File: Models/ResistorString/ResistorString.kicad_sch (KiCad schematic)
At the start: 3 parts

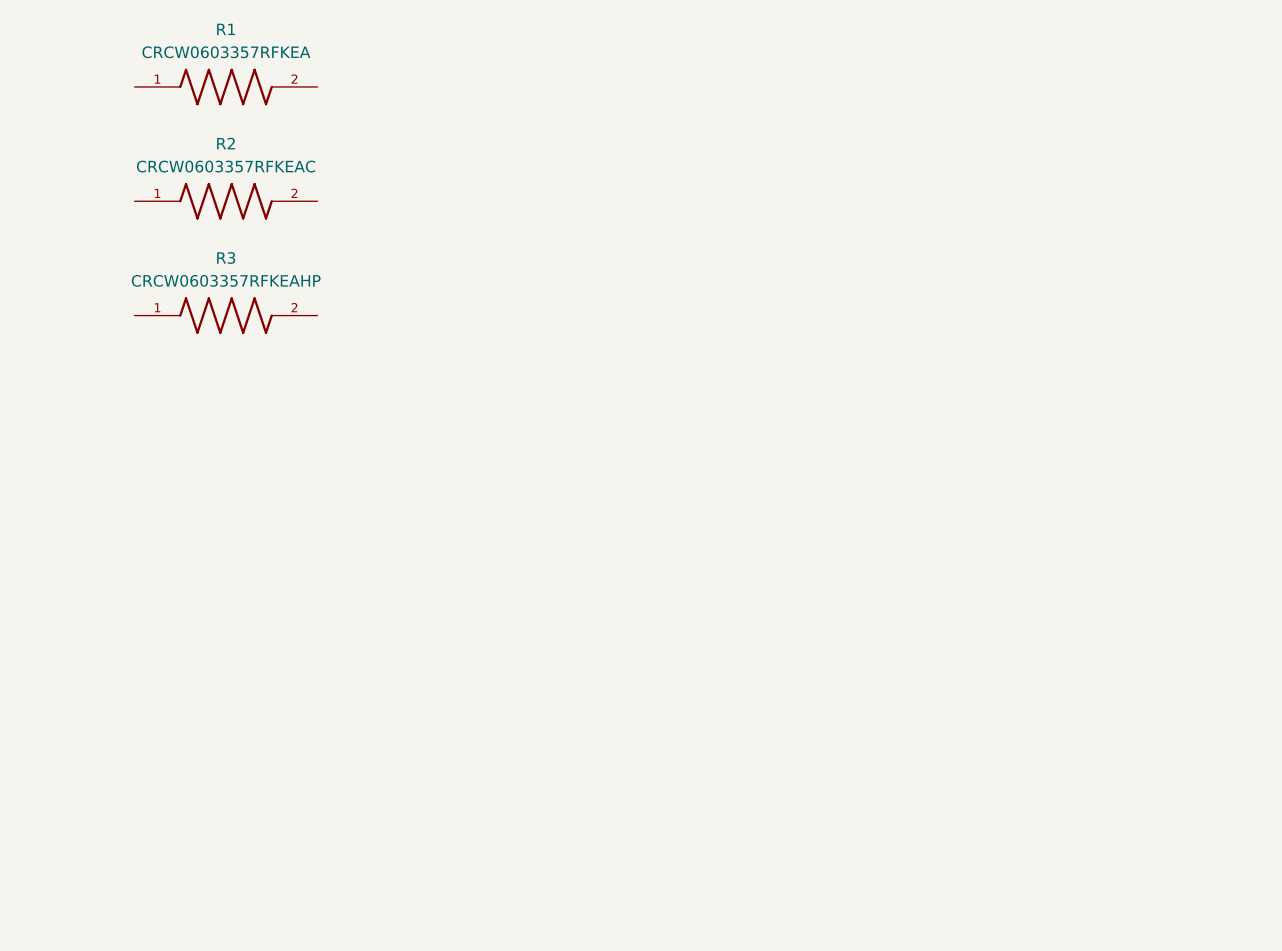
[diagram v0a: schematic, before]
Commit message: Upload modified KiCad project
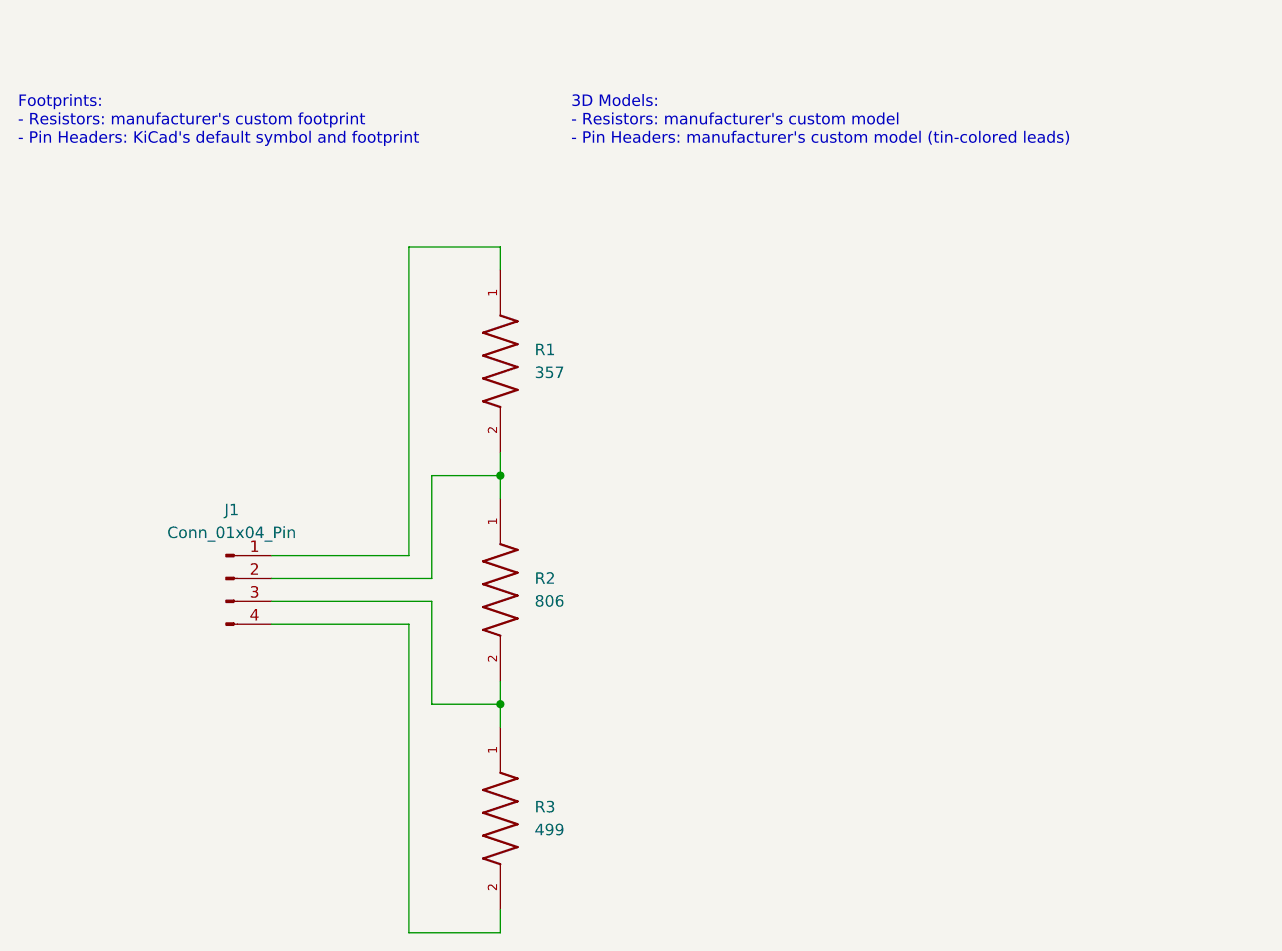
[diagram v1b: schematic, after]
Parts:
- removed R2: CRCW0603357RFKEAC, CRCW0603357RFKEAC:RESC1608X55N, symbol CRCW0603357RFKEAC:CRCW0603357RFKEAC
- removed R3: CRCW0603357RFKEAHP, CRCW0603357RFKEAHP:RESC1608X55N, symbol CRCW0603357RFKEAHP:CRCW0603357RFKEAHP
- added J1: Conn_01x04_Pin, Connector_PinHeader_2.54mm:PinHeader_1x04_P2.54mm_Vertical, symbol Connector:Conn_01x04_Pin
- added R2: 806, CRCW0603806RFKEA:RESC1508X50N, symbol CRCW0603806RFKEA:CRCW0603806RFKEA
- added R3: 499, CRCW0603499RFKEA:RESC1508X50N, symbol CRCW0603499RFKEA:CRCW0603499RFKEA
- R1: value CRCW0603357RFKEA -> 357; Price None -> $0.10; Purchase_Link (none) -> https://www.mouser.com/ProductDetail/Vishay-Dale/CRCW060335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
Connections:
- net at R1.1: now also J1.1 (Pin_1)
- net at R1.2: now also J1.2 (Pin_2), R2.1
- new net: J1.3 (Pin_3), R2.2, R3.1
- new net: J1.4 (Pin_4), R3.2
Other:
- note added: "3D Models: - Resistors: manufacturer's custom model - Pin Headers: manufacturer's custom model (tin-colored leads)"
- note added: "Footprints: - Resistors: manufacturer's custom footprint - Pin Headers: KiCad's default symbol and footprint"
